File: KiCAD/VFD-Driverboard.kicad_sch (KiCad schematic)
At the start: 16 parts, among them U1 MC34063AD, U2 LM4871MX_NOPB

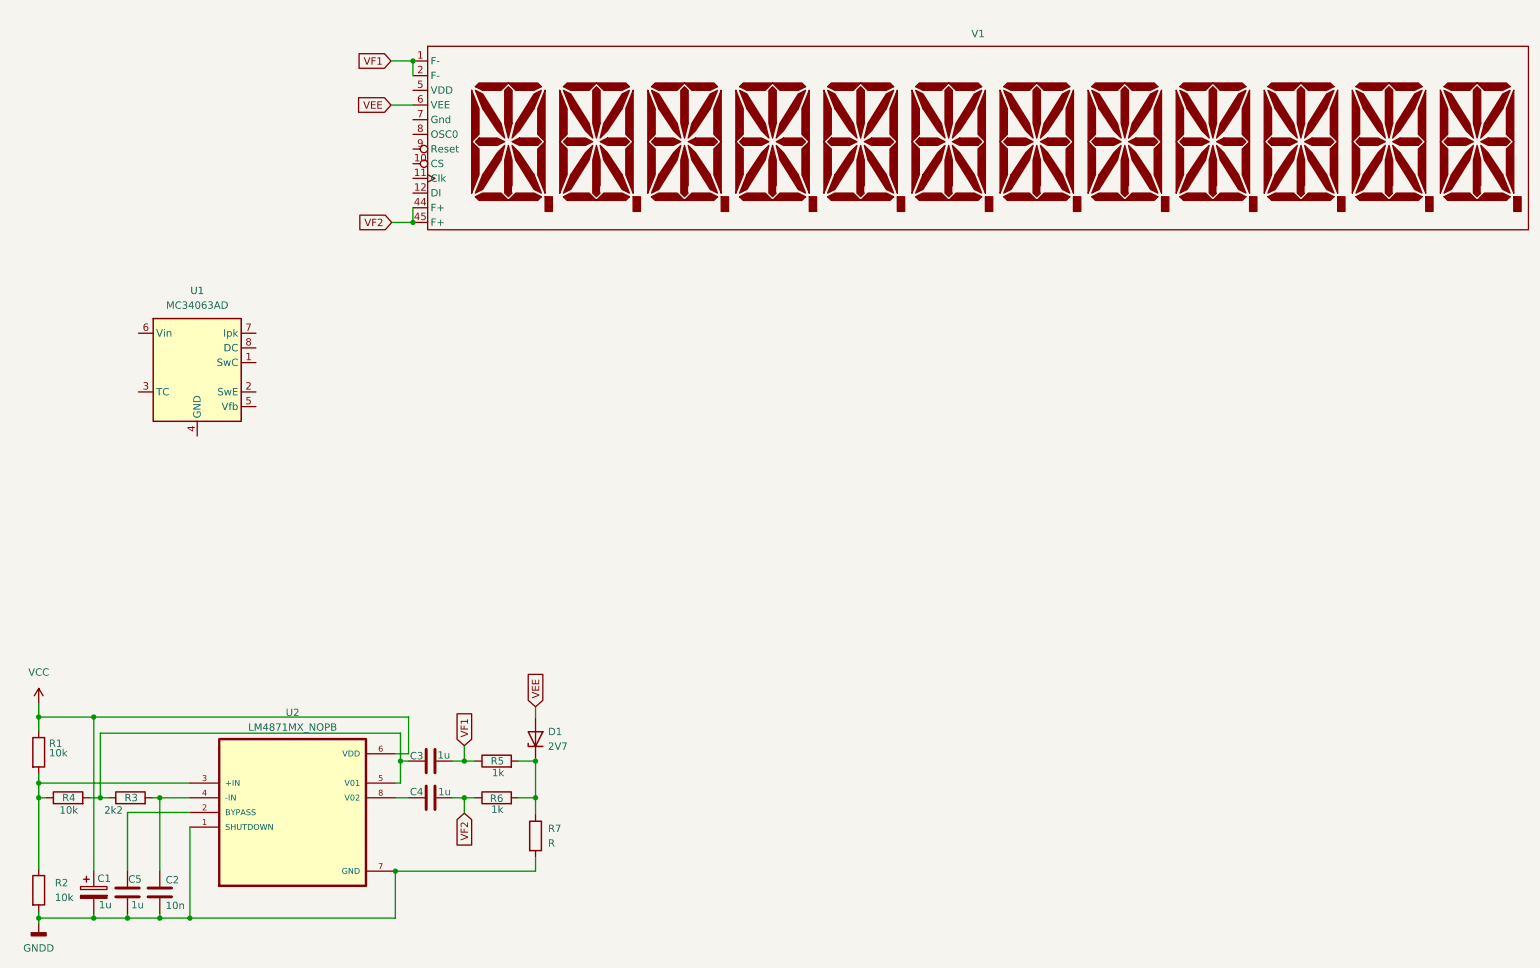
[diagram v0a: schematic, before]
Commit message: Driverboard v. 1.0.4
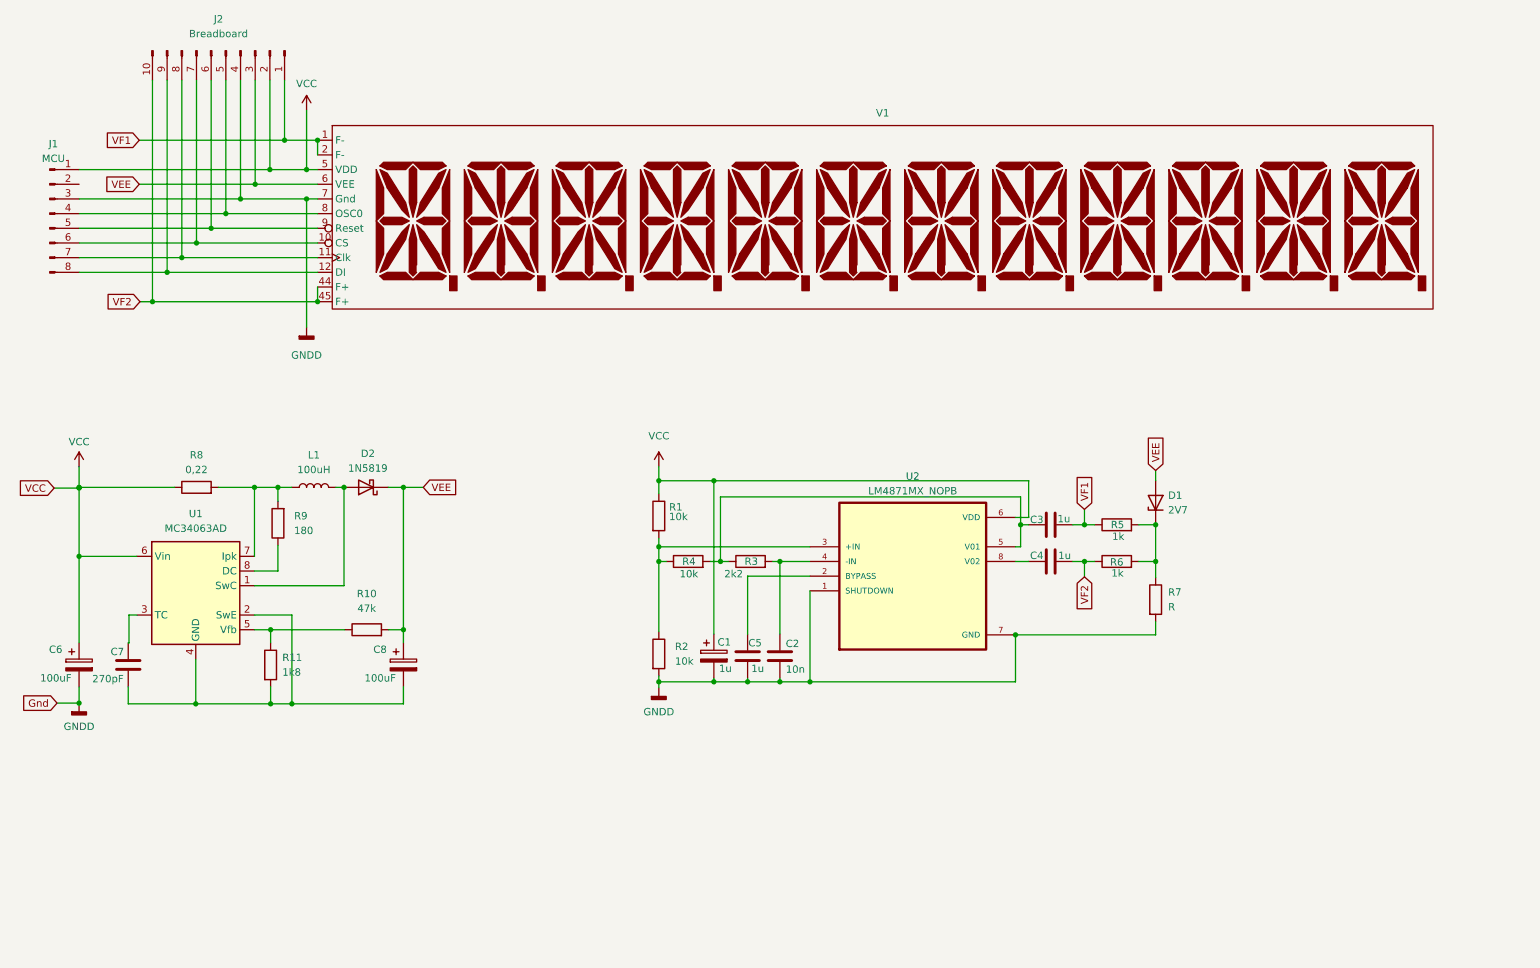
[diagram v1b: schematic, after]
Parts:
- added C6, C8: 100uF, Capacitor_THT:CP_Axial_L10.0mm_D4.5mm_P15.00mm_Horizontal, symbol Device:C_Polarized
- added C7: 270pF, Capacitor_THT:C_Disc_D4.3mm_W1.9mm_P5.00mm, symbol Device:C
- added D2: 1N5819, Diode_THT:D_DO-34_SOD68_P7.62mm_Horizontal, symbol Diode:1N5819
- added J1: MCU, Connector_PinSocket_2.54mm:PinSocket_1x08_P2.54mm_Vertical, symbol Connector:Conn_01x08_Pin
- added J2: Breadboard, Connector_PinHeader_2.54mm:PinHeader_1x10_P2.54mm_Vertical, symbol Connector:Conn_01x10_Pin
- added L1: 100uH, Inductor_THT:L_Axial_L5.3mm_D2.2mm_P2.54mm_Vertical_Vishay_IM-1, symbol Device:L
- added R10: 47k, Resistor_THT:R_Axial_DIN0207_L6.3mm_D2.5mm_P10.16mm_Horizontal, symbol Device:R
- added R11: 1k8, Resistor_THT:R_Axial_DIN0207_L6.3mm_D2.5mm_P10.16mm_Horizontal, symbol Device:R
- added R8: 0,22, Resistor_THT:R_Axial_DIN0204_L3.6mm_D1.6mm_P2.54mm_Vertical, symbol Device:R
- added R9: 180, Resistor_THT:R_Axial_DIN0207_L6.3mm_D2.5mm_P10.16mm_Horizontal, symbol Device:R
- C1, C2, C3, C4, C5: footprint Capacitor_SMD:C_1206_3216Metric_Pad1.33x1.80mm_HandSolder -> Capacitor_THT:C_Disc_D4.3mm_W1.9mm_P5.00mm
- D1: footprint Diode_SMD:D_1206_3216Metric_Pad1.42x1.75mm_HandSolder -> Diode_THT:D_DO-34_SOD68_P7.62mm_Horizontal
- R1, R2, R3, R4, R5, R6, R7: footprint Resistor_SMD:R_1206_3216Metric_Pad1.30x1.75mm_HandSolder -> Resistor_THT:R_Axial_DIN0207_L6.3mm_D2.5mm_P10.16mm_Horizontal
- U1, U2: footprint Package_SO:SOIC-8_3.9x4.9mm_P1.27mm -> Package_DIP:DIP-8_W7.62mm
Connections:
- net GNDD: now also V1.7 (Gnd), C6.2, J1.3 (Pin_3), J2.4 (Pin_4)
- net VCC: now also U1.6 (Vin), V1.5 (VDD), C6.1, J1.1 (Pin_1), J2.2 (Pin_2), R8.1
- net VEE: now also C8.1, D2.1 (K), J2.3 (Pin_3), R10.2
- net VF1: now also J2.1 (Pin_1)
- net VF2: now also J2.10 (Pin_10)
- net at V1.10 (CS): now also J1.6 (Pin_6), J2.7 (Pin_7)
- net at V1.11 (Clk): now also J1.7 (Pin_7), J2.8 (Pin_8)
- net at V1.12 (DI): now also J1.8 (Pin_8), J2.9 (Pin_9)
- net at V1.8 (OSC0): now also J1.4 (Pin_4), J2.5 (Pin_5)
- net at V1.9 (Reset): now also J1.5 (Pin_5), J2.6 (Pin_6)
- net at U1.1 (SwC): now also D2.2 (A), L1.2
- net at U1.2 (SwE): now also U1.4 (GND), C7.2, C8.2, R11.2
- net at U1.3 (TC): now also C7.1
- net at U1.5 (Vfb): now also R10.1, R11.1
- net at U1.7 (Ipk): now also L1.1, R8.2, R9.2
- net at U1.8 (DC): now also R9.1
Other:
- company: (none) -> (C) Karl
- title: (none) -> VFD driver board HCS-12SS59T
- moved on the sheet: C1, C2, C3, C4, C5, D1, R1, R2, R3, R4, R5, R6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
